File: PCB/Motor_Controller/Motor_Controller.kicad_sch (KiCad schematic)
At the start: 6 parts, among them J1 Motor, Q1 FQD50N06

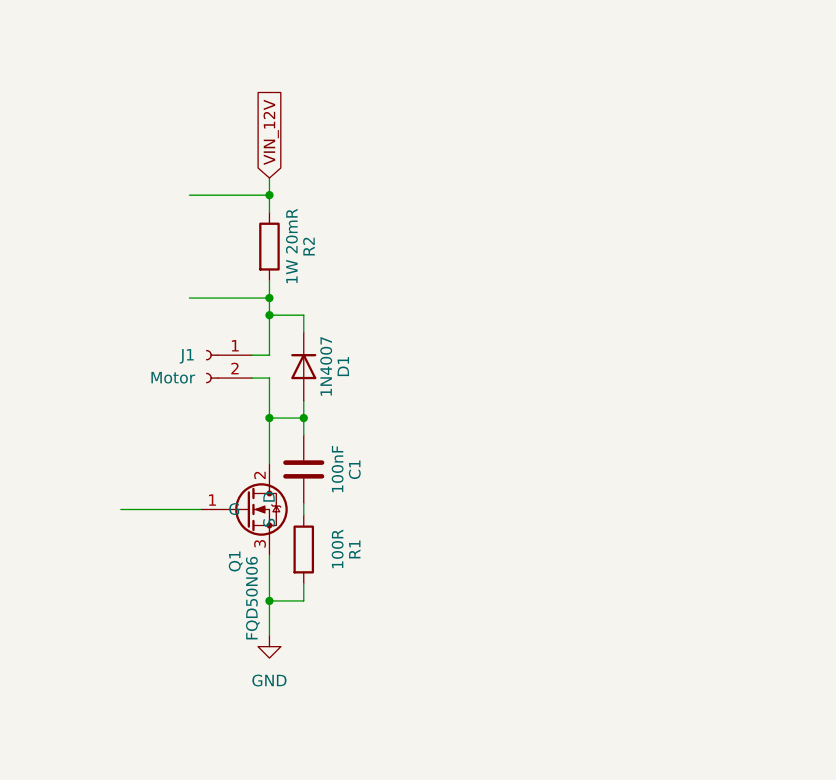
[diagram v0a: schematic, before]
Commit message: PCB and PWM Update
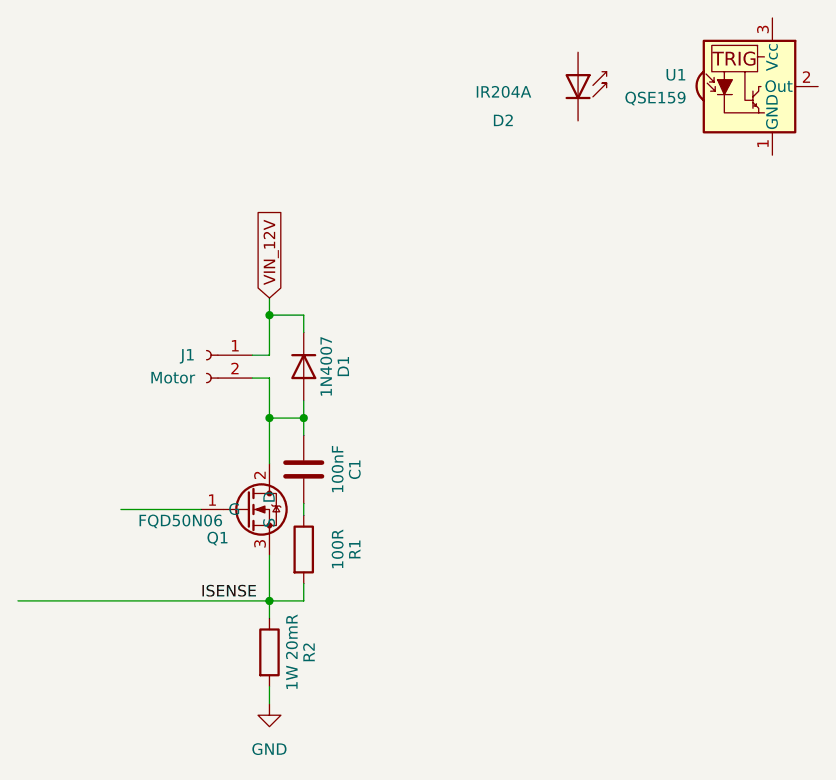
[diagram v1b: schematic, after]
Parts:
- added D2: IR204A, LED_THT:LED_D3.0mm_IRBlack, symbol LED:IR204A
- added U1: QSE159, OptoDevice:ONSemi_QSE15x, symbol Interface_Optical:QSE159
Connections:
- net GND: now also R2.2; no longer Q1.3 (S), R1.2
- net VIN_12V: now also D1.1 (K), J1.1 (Pin_1); no longer R2.1
- new net ISENSE: Q1.3 (S), R1.2, R2.1
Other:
- moved on the sheet: R2
